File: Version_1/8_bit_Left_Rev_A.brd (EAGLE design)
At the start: 146.8 x 162.6 mm, 164 parts, among them IC1 74LS157N, IC10 74LS08N, IC11 74LS32N, IC12 74LS04N, IC13 7404N, IC14 74157N, IC15 7400N, IC16 74LS173N, IC17 74LS173N, IC18 74LS245N, IC2 74LS173N, IC25 74LS138N, IC26 28C16AP, IC27 28C16AP, IC28 7404N, IC3 74157N, IC39 7404N, IC4 74157N, IC40 7400N, IC5 74LS245N, IC6 LM555N, IC7 7404N, IC8 LM555N, IC9 LM555N, SW2 , SW3 , U1 74LS161N

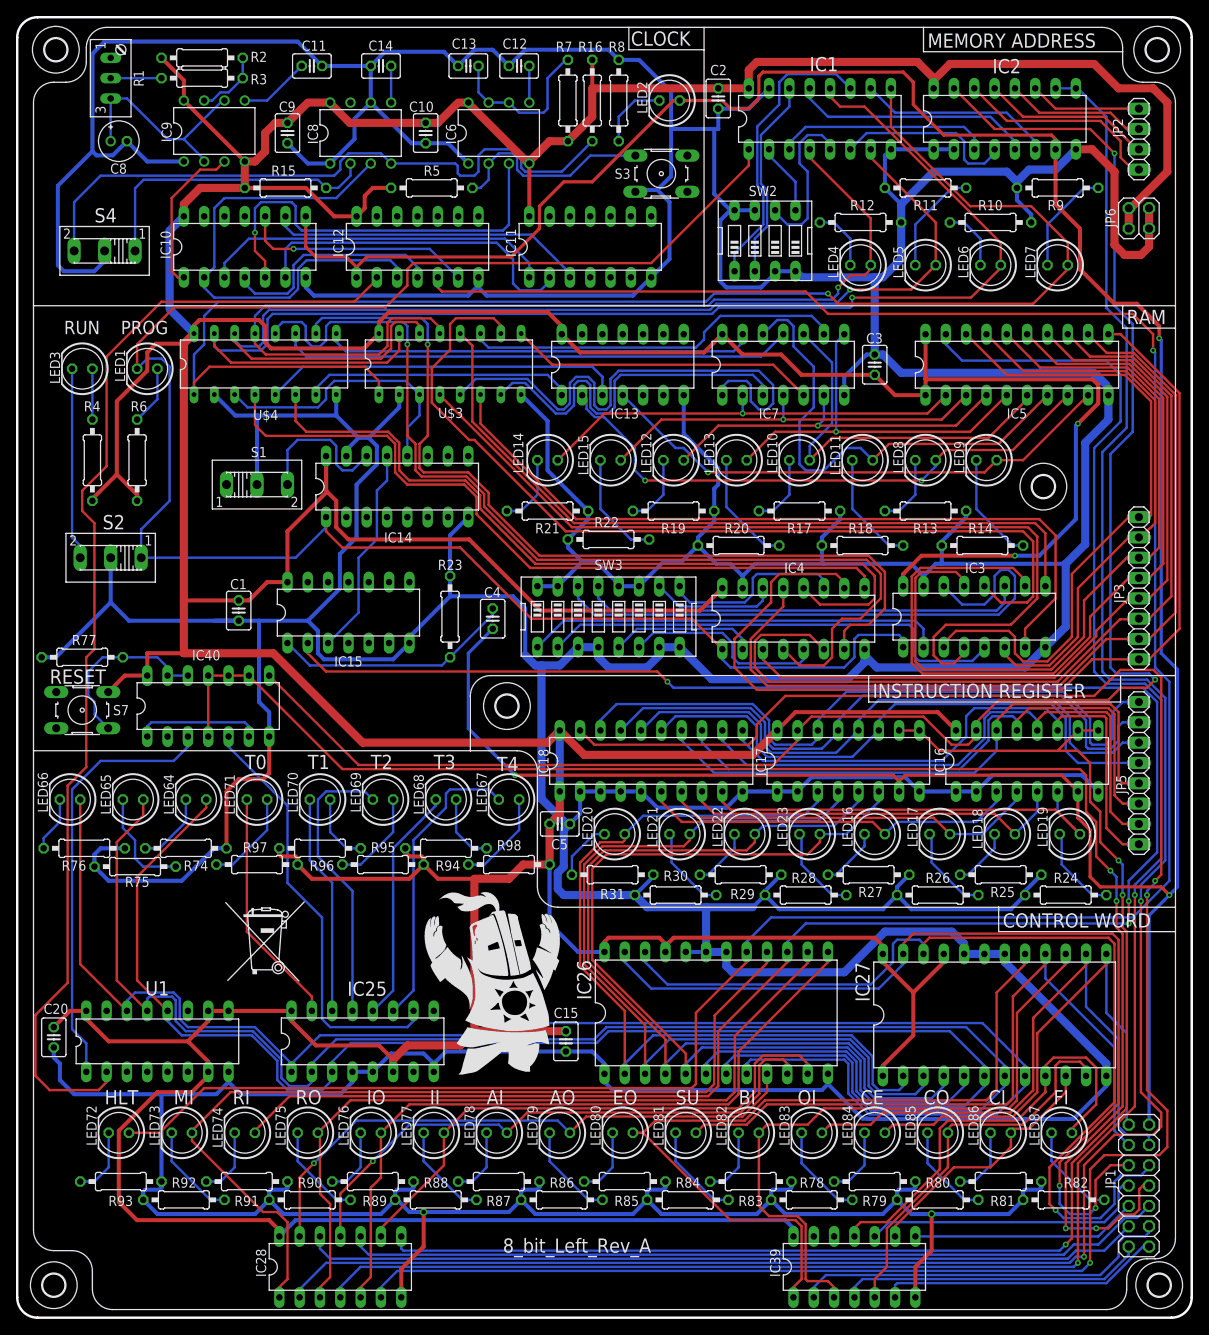
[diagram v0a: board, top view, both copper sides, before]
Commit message: Fixed DRC problems
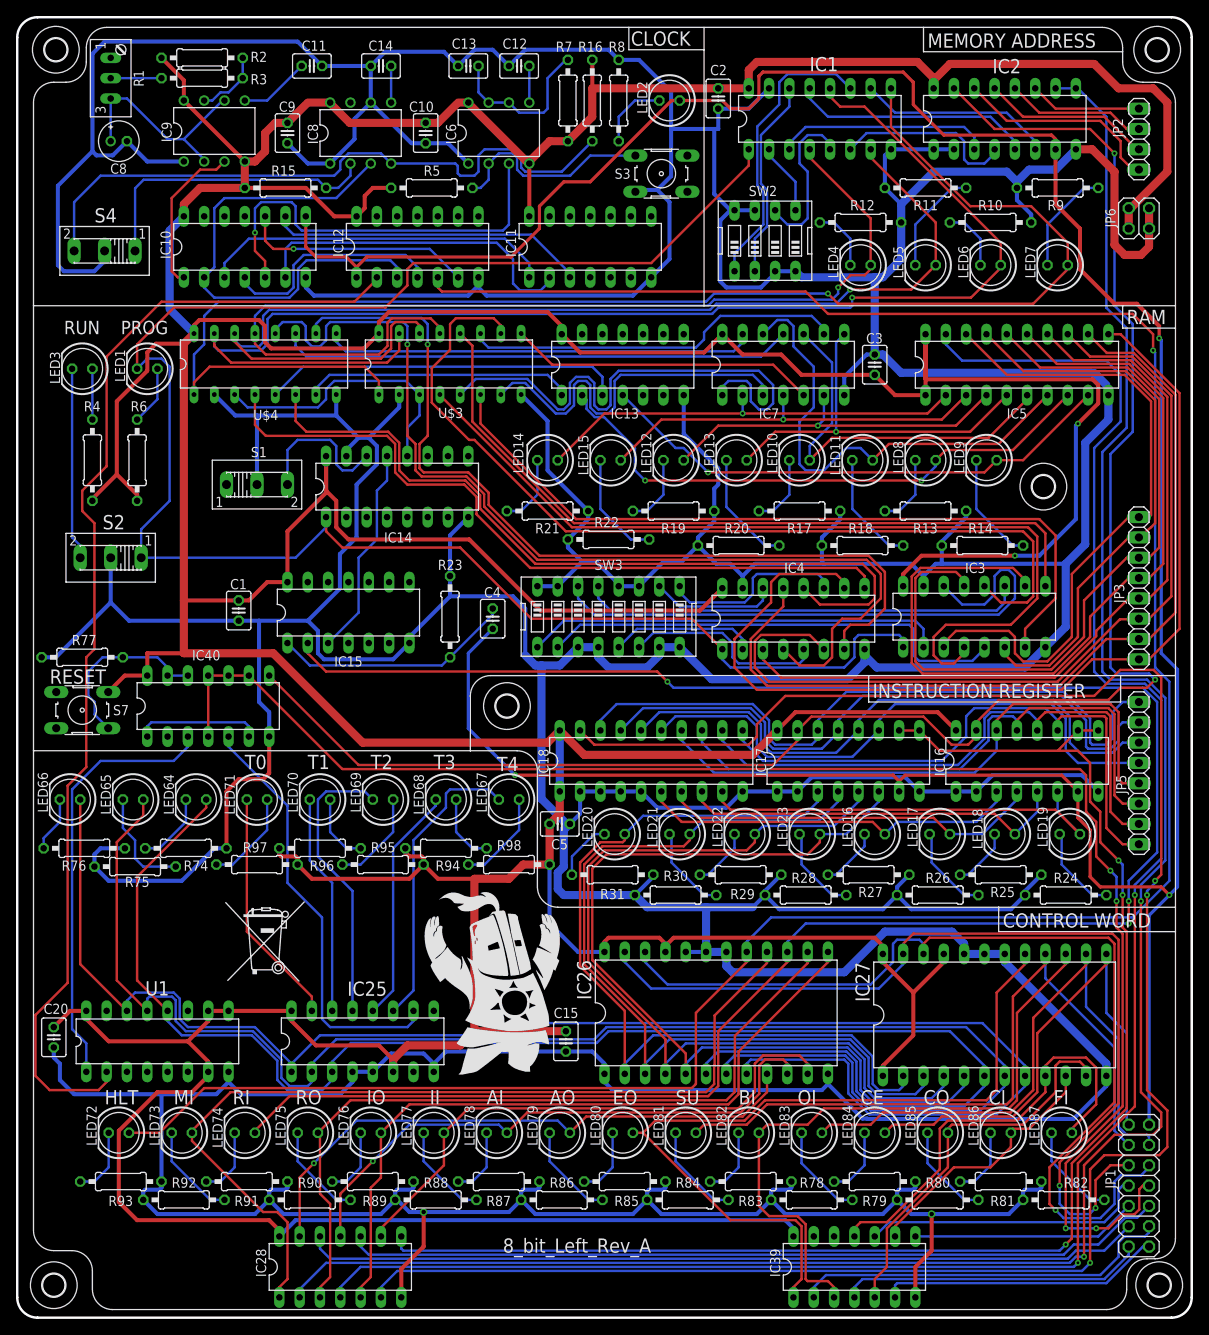
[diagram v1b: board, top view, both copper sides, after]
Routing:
- net GND: track 1509.7 -> 1503.5 mm
- net VCC: track 1073.4 -> 1078.5 mm
- net N$34: track 43.1 -> 42.1 mm
- net N$11: track 24.8 -> 24.3 mm
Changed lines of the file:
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@@
 <wire x1="54.102" y1="92.71" x2="54.102" y2="97.79" width="0.508" layer="16"/>
 <wire x1="54.102" y1="97.79" x2="56.388" y2="100.076" width="0.508" layer="16"/>
-<wire x1="24.6888" y1="87.122" x2="27.686" y2="87.122" width="0.508" layer="16"/>
 <wire x1="40.3352" y1="95.4532" x2="42.418" y2="97.536" width="0.508" layer="16"/>
 <wire x1="42.418" y1="97.536" x2="42.418" y2="104.14" width="0.508" layer="16"/>
@@
 <wire x1="93.472" y1="53.34" x2="95.504" y2="55.372" width="0.508" layer="16"/>
 <wire x1="91.948" y1="51.308" x2="93.472" y2="52.832" width="0.508" layer="16"/>
-<wire x1="135.128" y1="65.786" x2="135.382" y2="65.532" width="0.508" layer="16"/>
 <wire x1="135.128" y1="65.786" x2="133.096" y2="67.818" width="0.508" layer="16"/>
 <wire x1="121.92" y1="67.818" x2="119.888" y2="65.786" width="0.508" layer="16"/>
@@
 <wire x1="80.01" y1="63.754" x2="88.646" y2="63.754" width="0.508" layer="16"/>
 <wire x1="70.358" y1="65.786" x2="70.358" y2="62.992" width="0.508" layer="16"/>
-<wire x1="77.216" y1="52.832" x2="77.216" y2="53.086" width="0.508" layer="16"/>
 <wire x1="79.502" y1="55.118" x2="77.216" y2="52.832" width="0.508" layer="16"/>
 <wire x1="79.502" y1="55.118" x2="79.502" y2="55.372" width="0.508" layer="16"/>
@@
 <wire x1="61.468" y1="13.208" x2="50.8" y2="13.208" width="0.508" layer="16"/>
 <wire x1="86.106" y1="45.72" x2="83.566" y2="45.72" width="0.508" layer="16"/>
-<wire x1="118.364" y1="46.482" x2="118.364" y2="45.466" width="0.508" layer="16"/>
 <wire x1="101.346" y1="29.21" x2="100.584" y2="28.448" width="0.508" layer="16"/>
 <wire x1="73.406" y1="29.464" x2="73.406" y2="30.48" width="0.508" layer="16"/>
@@
 <wire x1="11.684" y1="89.408" x2="4.826" y2="82.55" width="0.508" layer="16"/>
 <wire x1="11.684" y1="89.408" x2="13.97" y2="87.122" width="0.508" layer="16"/>
-<wire x1="13.97" y1="87.122" x2="27.686" y2="87.122" width="0.508" layer="16"/>
+<wire x1="27.686" y1="87.122" x2="13.97" y2="87.122" width="0.508" layer="16"/>
 <wire x1="30.226" y1="87.122" x2="30.226" y2="76.962" width="0.508" layer="16"/>
 <wire x1="30.226" y1="76.962" x2="31.496" y2="75.692" width="0.508" layer="16"/>
@@
 <wire x1="26.162" y1="65.786" x2="27.686" y2="67.31" width="0.508" layer="1"/>
 <wire x1="30.734" y1="67.31" x2="27.686" y2="67.31" width="0.508" layer="1"/>
-<wire x1="24.638" y1="115.396" x2="27.258" y2="112.776" width="0.508" layer="16"/>
-<wire x1="27.258" y1="112.776" x2="29.972" y2="112.776" width="0.508" layer="16"/>
+<wire x1="29.972" y1="112.776" x2="27.258" y2="112.776" width="0.508" layer="16"/>
 <wire x1="29.972" y1="112.776" x2="39.878" y2="112.776" width="0.508" layer="16"/>
 <wire x1="75.184" y1="157.226" x2="77.724" y2="157.226" width="0.508" layer="16"/>
@@
 <wire x1="87.122" y1="148.59" x2="87.63" y2="148.59" width="0.508" layer="16"/>
 <wire x1="11.684" y1="94.996" x2="11.684" y2="89.408" width="0.508" layer="16"/>
-<wire x1="29.972" y1="105.664" x2="29.972" y2="104.14" width="0.508" layer="16"/>
-<wire x1="29.972" y1="104.14" x2="29.972" y2="112.776" width="0.508" layer="16"/>
+<wire x1="29.972" y1="112.776" x2="29.972" y2="104.14" width="0.508" layer="16"/>
 <wire x1="67.818" y1="81.534" x2="65.532" y2="81.534" width="1.016" layer="16"/>
 <wire x1="65.532" y1="81.534" x2="64.77" y2="81.534" width="1.016" layer="16"/>
@@
 <wire x1="9.652" y1="57.912" x2="10.414" y2="58.674" width="0.508" layer="16"/>
 <wire x1="10.414" y1="58.674" x2="13.462" y2="58.674" width="0.508" layer="16"/>
+<wire x1="27.258" y1="112.776" x2="24.638" y2="115.396" width="0.508" layer="16"/>
 </signal>
 <signal name="VCC" class="1">
@@
 <wire x1="45.212" y1="123.016" x2="45.212" y2="124.46" width="0.508" layer="1"/>
 <wire x1="68.072" y1="123.952" x2="66.294" y2="125.73" width="0.508" layer="1"/>
-<wire x1="113.538" y1="115.316" x2="113.538" y2="115.824" width="0.508" layer="1"/>
 <wire x1="135.128" y1="116.586" x2="134.4168" y2="117.2972" width="0.508" layer="1"/>
 <wire x1="135.128" y1="114.3" x2="132.588" y2="111.76" width="0.508" layer="1"/>
@@
 <wire x1="90.678" y1="120.396" x2="95.504" y2="120.396" width="0.508" layer="1"/>
 <wire x1="113.538" y1="122.936" x2="113.538" y2="117.348" width="0.508" layer="1"/>
-<wire x1="113.538" y1="117.348" x2="113.538" y2="115.316" width="0.508" layer="1"/>
+<wire x1="113.538" y1="122.936" x2="113.538" y2="115.316" width="0.508" layer="1"/>
 <wire x1="113.5888" y1="117.2972" x2="113.538" y2="117.348" width="0.508" layer="1"/>
 <wire x1="134.4168" y1="117.2972" x2="113.5888" y2="117.2972" width="0.508" layer="1"/>
@@
 <contactref element="IC10" pad="6"/>
 <contactref element="IC11" pad="2"/>
-<wire x1="66.548" y1="130.048" x2="66.548" y2="131.064" width="0.3048" layer="16"/>
 <wire x1="66.548" y1="130.048" x2="66.548" y2="129.54" width="0.3048" layer="16"/>
 <wire x1="65.4304" y1="128.4224" x2="62.8396" y2="128.4224" width="0.3048" layer="16"/>
@@
 <wire x1="65.278" y1="136.144" x2="65.278" y2="138.938" width="0.4064" layer="1"/>
 <wire x1="65.278" y1="138.938" x2="68.326" y2="141.986" width="0.4064" layer="1"/>
-<wire x1="68.326" y1="141.986" x2="71.882" y2="141.986" width="0.4064" layer="1"/>
-<wire x1="82.042" y1="152.146" x2="82.804" y2="152.146" width="0.4064" layer="1"/>
-<wire x1="82.042" y1="152.146" x2="71.882" y2="141.986" width="0.4064" layer="1"/>
+<wire x1="68.326" y1="141.986" x2="71.628" y2="141.986" width="0.4064" layer="1"/>
+<wire x1="81.788" y1="152.146" x2="82.804" y2="152.146" width="0.4064" layer="1"/>
+<wire x1="81.788" y1="152.146" x2="71.628" y2="141.986" width="0.4064" layer="1"/>
 <wire x1="82.804" y1="152.146" x2="88.138" y2="152.146" width="0.4064" layer="1"/>
 <wire x1="88.138" y1="152.146" x2="89.154" y2="151.13" width="0.4064" layer="1"/>
@@
 <contactref element="IC1" pad="10"/>
 <contactref element="IC2" pad="6"/>
-<wire x1="106.68" y1="153.67" x2="106.68" y2="153.162" width="0.3048" layer="16"/>
 <wire x1="127.254" y1="147.066" x2="127.254" y2="146.05" width="0.3048" layer="16"/>
 <wire x1="123.698" y1="150.622" x2="127.254" y2="147.066" width="0.3048" layer="16"/>
